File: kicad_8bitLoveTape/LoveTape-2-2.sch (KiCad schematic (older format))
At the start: 13 parts, among them J1 audio out, SW3 On-Off, U1 ATTINY85-20PU

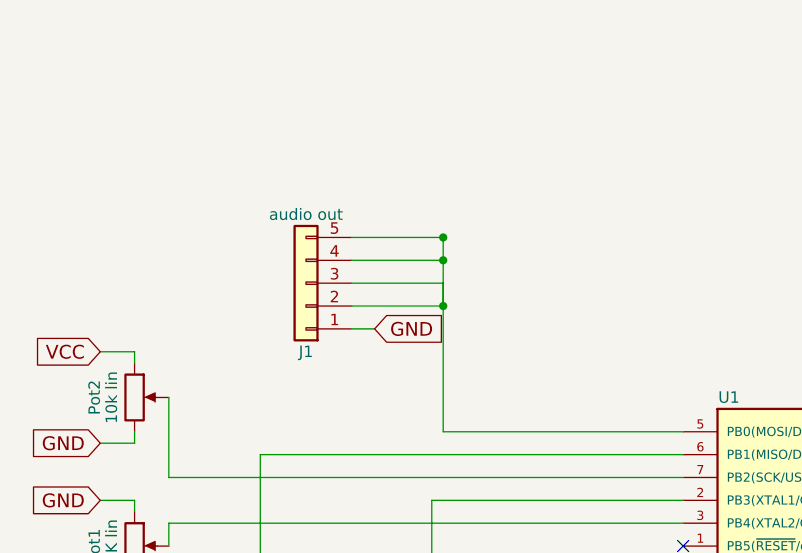
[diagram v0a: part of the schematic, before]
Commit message: fix some bad routings...
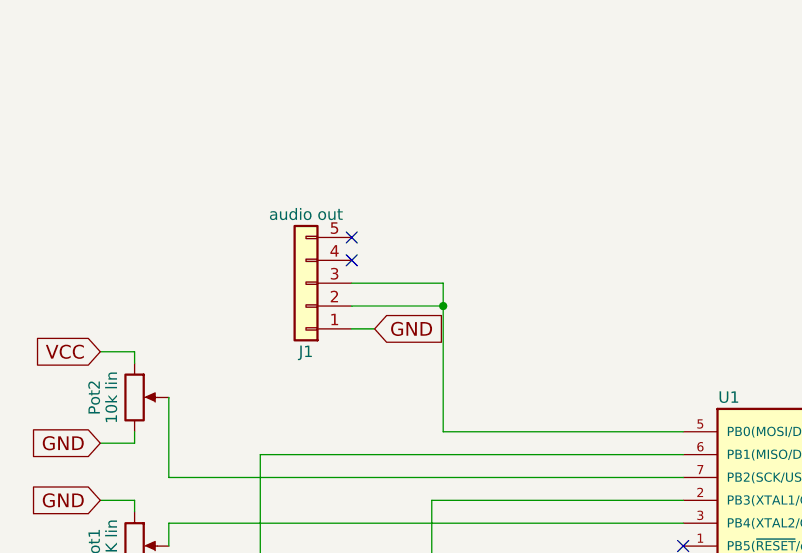
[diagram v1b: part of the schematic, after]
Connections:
- net at J1.2 (Pin_2), J1.3 (Pin_3), U1.5 (PB0(MOSI/DI/SDA/AIN0/OC0A/OC1A/AREF/PCINT0)): no longer J1.4 (Pin_4), J1.5 (Pin_5)
- no-connect marks 2 -> 4
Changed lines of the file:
@@
 	5250 3150 4850 3150
-Wire Wire Line
-	4850 2950 5250 2950
-Wire Wire Line
-	5250 2850 5250 3150
-Connection ~ 5250 2950
-Connection ~ 5250 2850
 Wire Wire Line
 	9200 3300 9200 3600
@@
 	5250 3700 6300 3700
 NoConn ~ 6300 4200
-Wire Wire Line
-	4850 2850 5250 2850
+NoConn ~ 4850 2950
+NoConn ~ 4850 2850
 $EndSCHEMATC
